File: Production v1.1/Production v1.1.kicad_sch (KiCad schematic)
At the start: 28 parts, among them IC1 MAX3323EEUE+T, IC2 AP7375-33SA-7, J1 530480510, J2 530480410, J3 USB4085-GF-A_REVB, U2 ADR02AUJZ-REEL7, U3 ATSAMD21G18A-AUT, Y1 32.768, 12.5pF

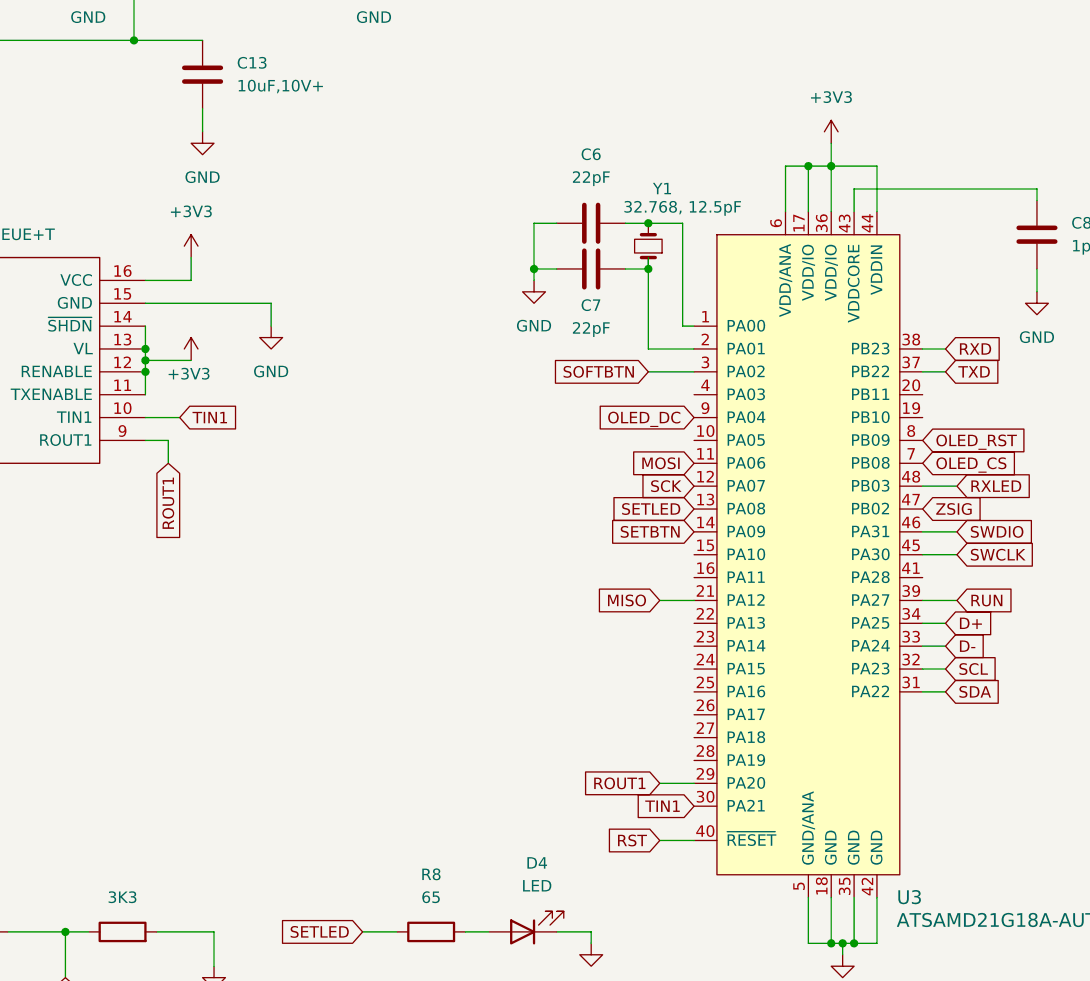
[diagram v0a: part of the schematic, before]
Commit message: Solid v1.1 attempt, but going to start over
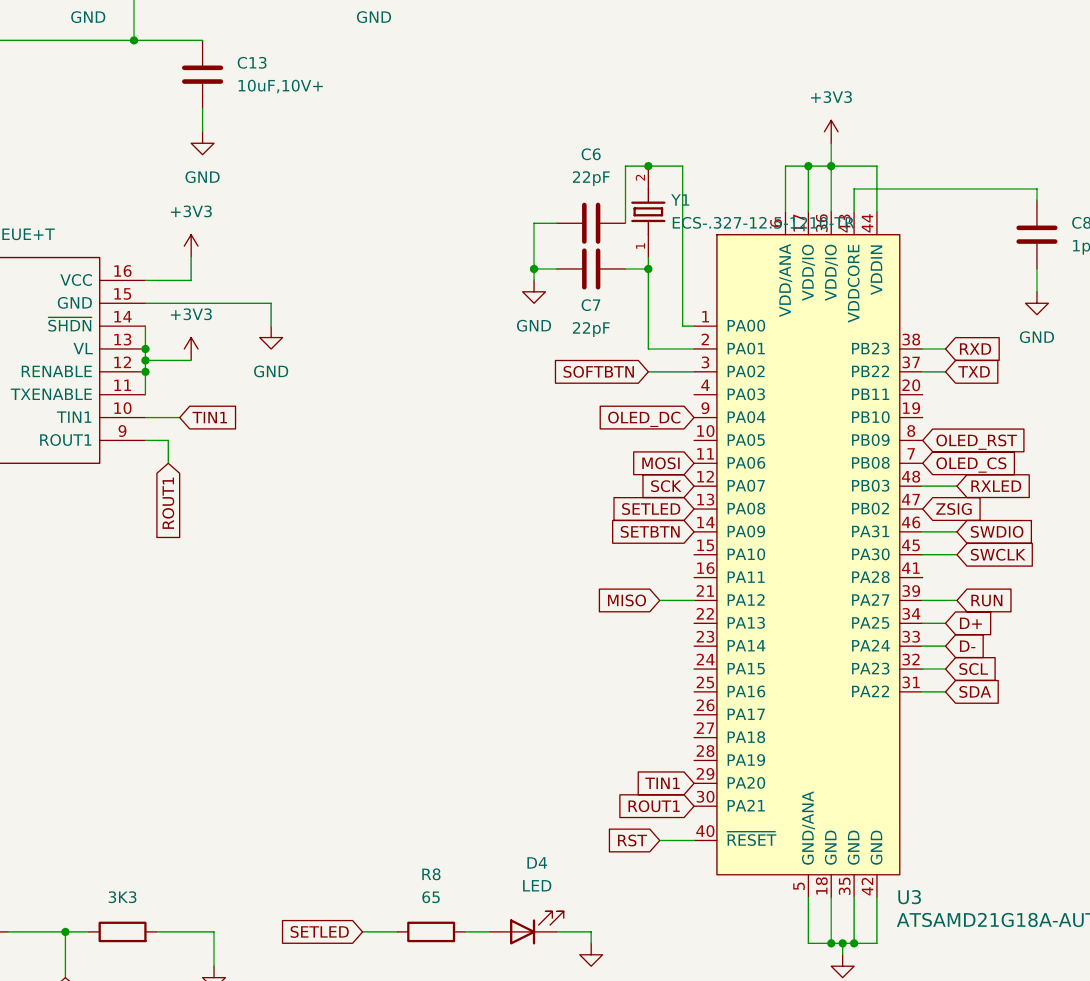
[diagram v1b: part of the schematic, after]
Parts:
- removed Y1: 32.768, 12.5pF, Crystal:Crystal_SMD_3215-2Pin_3.2x1.5mm, symbol Device:Crystal_Small
- added Y1: ECS-.327-12.5-1210-TR, ECS__327_12_5_1210_TR:XTAL_ECS-.327-12.5-1210-TR, symbol ECS-.327-12.5-1210-TR:ECS-.327-12.5-1210-TR
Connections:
- net ROUT1: now also U3.30 (PA21); no longer U3.29 (PA20)
- net TIN1: now also U3.29 (PA20); no longer U3.30 (PA21)
- net at C6.2, U3.1 (PA00): now also Y1.2
- net at C7.2, U3.2 (PA01): now also Y1.1
